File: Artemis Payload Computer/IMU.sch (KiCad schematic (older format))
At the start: 1 part, among them U401 FXOS8700+FXAS21002

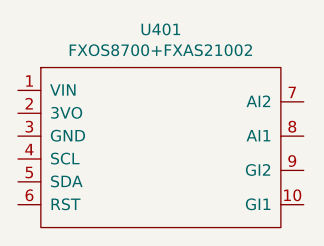
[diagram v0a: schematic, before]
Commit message: I think I undid this...
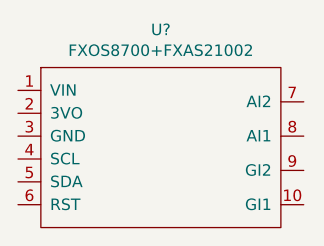
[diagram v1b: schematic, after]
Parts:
- renumbered U401 to U?
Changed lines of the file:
@@
 $Descr A4 11693 8268
 encoding utf-8
-Sheet 4 5
+Sheet 4 4
 Title ""
 Date ""
@@
 $EndDescr
 $Comp
-L Artemis_Footprints:FXOS8700+FXAS21002 U401
+L Artemis_Footprints:FXOS8700+FXAS21002 U?
 U 1 1 603A9652
 P 6250 3450
-F 0 "U401" H 6275 3965 50  0000 C CNN
+F 0 "U?" H 6275 3965 50  0000 C CNN
 F 1 "FXOS8700+FXAS21002" H 6275 3874 50  0000 C CNN
 F 2 "" H 6250 3450 50  0001 C CNN

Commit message: Fuck it we're starting over. Sorry for the mess Nathan
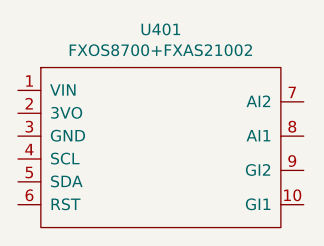
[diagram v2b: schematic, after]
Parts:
- gave numbers to parts that had none: 1
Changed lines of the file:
@@
 $Descr A4 11693 8268
 encoding utf-8
-Sheet 4 4
+Sheet 4 5
 Title ""
 Date ""
@@
 $EndDescr
 $Comp
-L Artemis_Footprints:FXOS8700+FXAS21002 U?
+L Artemis_Footprints:FXOS8700+FXAS21002 U401
 U 1 1 603A9652
 P 6250 3450
-F 0 "U?" H 6275 3965 50  0000 C CNN
+F 0 "U401" H 6275 3965 50  0000 C CNN
 F 1 "FXOS8700+FXAS21002" H 6275 3874 50  0000 C CNN
 F 2 "" H 6250 3450 50  0001 C CNN

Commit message: complete redo hehe
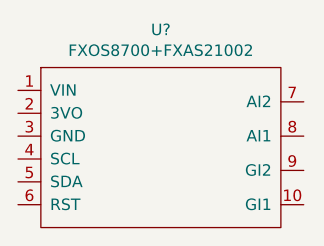
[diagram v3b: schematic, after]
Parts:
- U?: renamed from U401; footprint (none) -> Artemis Payload Computer:IMU
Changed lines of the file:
@@
 $Descr A4 11693 8268
 encoding utf-8
-Sheet 4 5
+Sheet 4 6
 Title ""
 Date ""
@@
 $EndDescr
 $Comp
-L Artemis_Footprints:FXOS8700+FXAS21002 U401
+L Artemis_Footprints:FXOS8700+FXAS21002 U?
 U 1 1 603A9652
 P 6250 3450
-F 0 "U401" H 6275 3965 50  0000 C CNN
+F 0 "U?" H 6275 3965 50  0000 C CNN
 F 1 "FXOS8700+FXAS21002" H 6275 3874 50  0000 C CNN
-F 2 "" H 6250 3450 50  0001 C CNN
+F 2 "Artemis Payload Computer:IMU" H 6250 3450 50  0001 C CNN
 F 3 "" H 6250 3450 50  0001 C CNN
 	1    6250 3450
